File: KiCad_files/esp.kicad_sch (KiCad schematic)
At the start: 18 parts, among them J2 USB_C_Receptacle_USB2.0_16P, Q1 DMP3099L, SW1 SW_Push, U1 ESP32-S3-MINI-1U, U2 BNO085, U6 LTC4412xS6

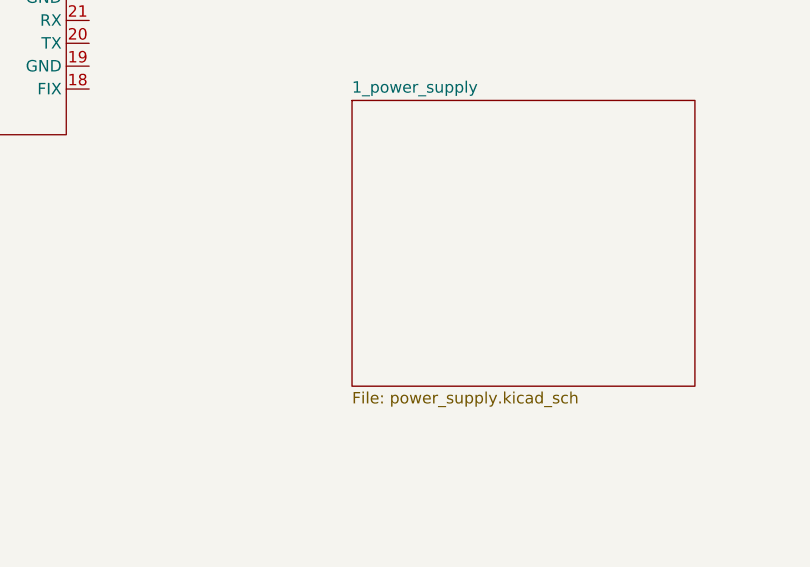
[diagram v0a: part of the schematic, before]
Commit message: hierarkiset pinnit poweriin
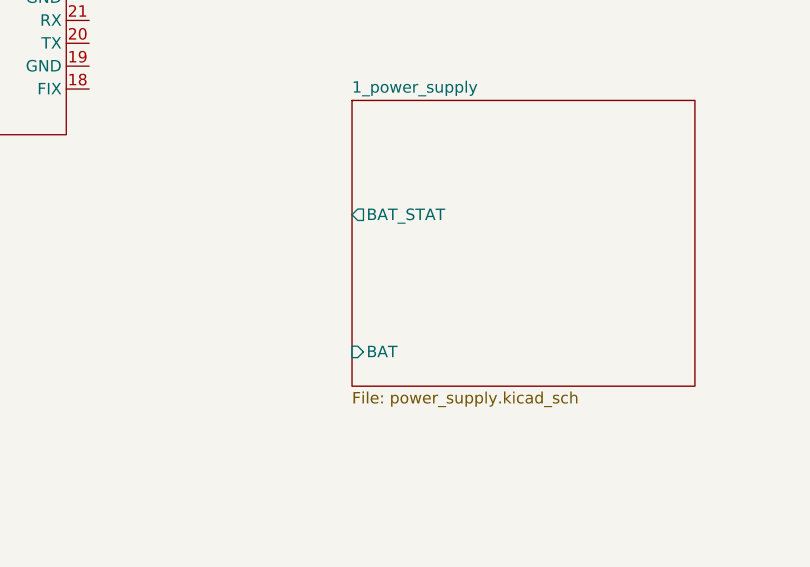
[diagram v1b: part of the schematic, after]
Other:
- sheet 1_power_supply ports: added BAT, BAT_STAT; removed none
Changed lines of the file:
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@@
+			)
+		)
+		(pin "BAT" input
+			(at 256.54 119.38 180)
+			(effects
+				(font
+					(size 1.27 1.27)
+				)
+				(justify left)
+			)
+		)
+		(pin "BAT_STAT" output
+			(at 256.54 104.14 180)
+			(effects
+				(font
+					(size 1.27 1.27)
+				)
+				(justify left)
 			)
 		)
